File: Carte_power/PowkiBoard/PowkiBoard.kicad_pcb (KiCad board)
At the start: 4 copper layers, 74.5 x 85.5 mm, 117 parts, among them J1 AUConn, J2 VBATT, J3 GNDBATT, J4 POW_strat, J5 POW_motors, J6 POW_Access, J7 POW_access, J8 SWLogic, J9 POW_EN, Q2 DMG1012T, Q3 DMG1012T, Q4 DMG1012T, Q5 DMG1012T

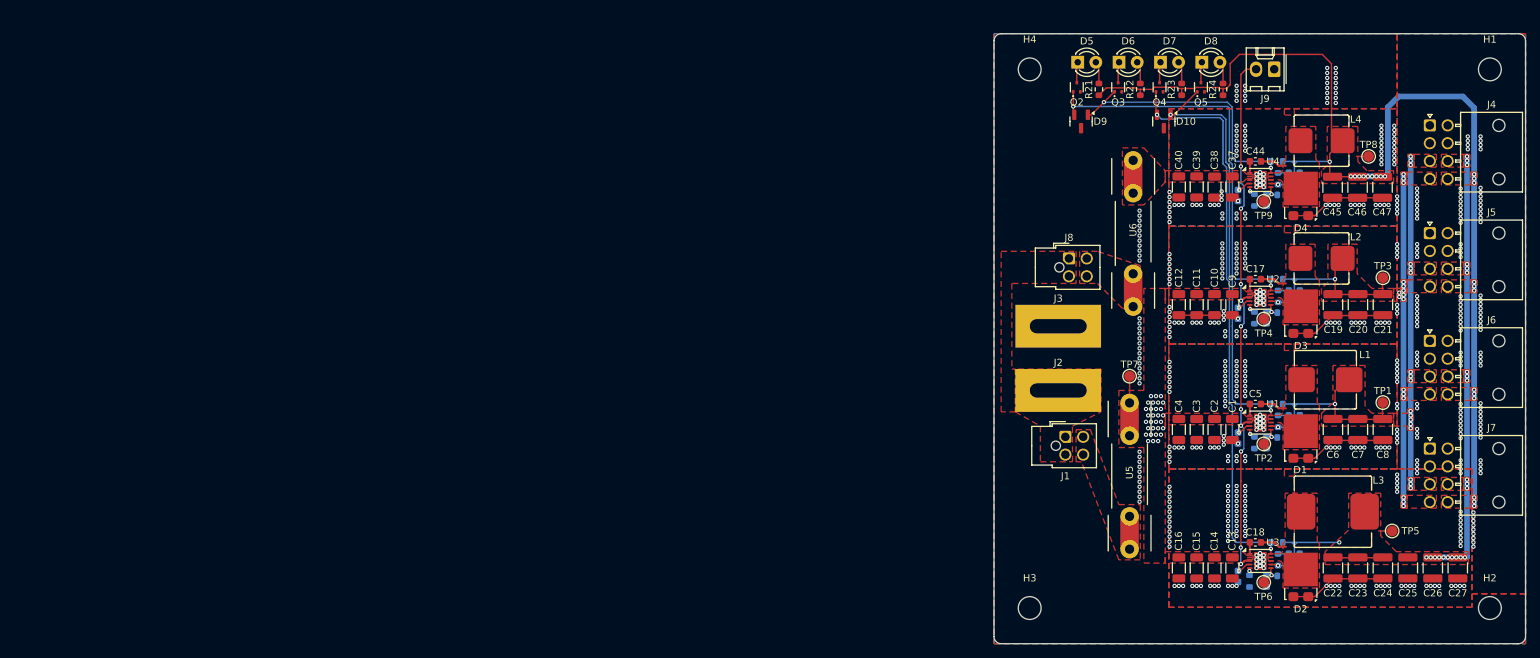
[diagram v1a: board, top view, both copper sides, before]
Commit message: AAAAAAAAAAAAAAAA
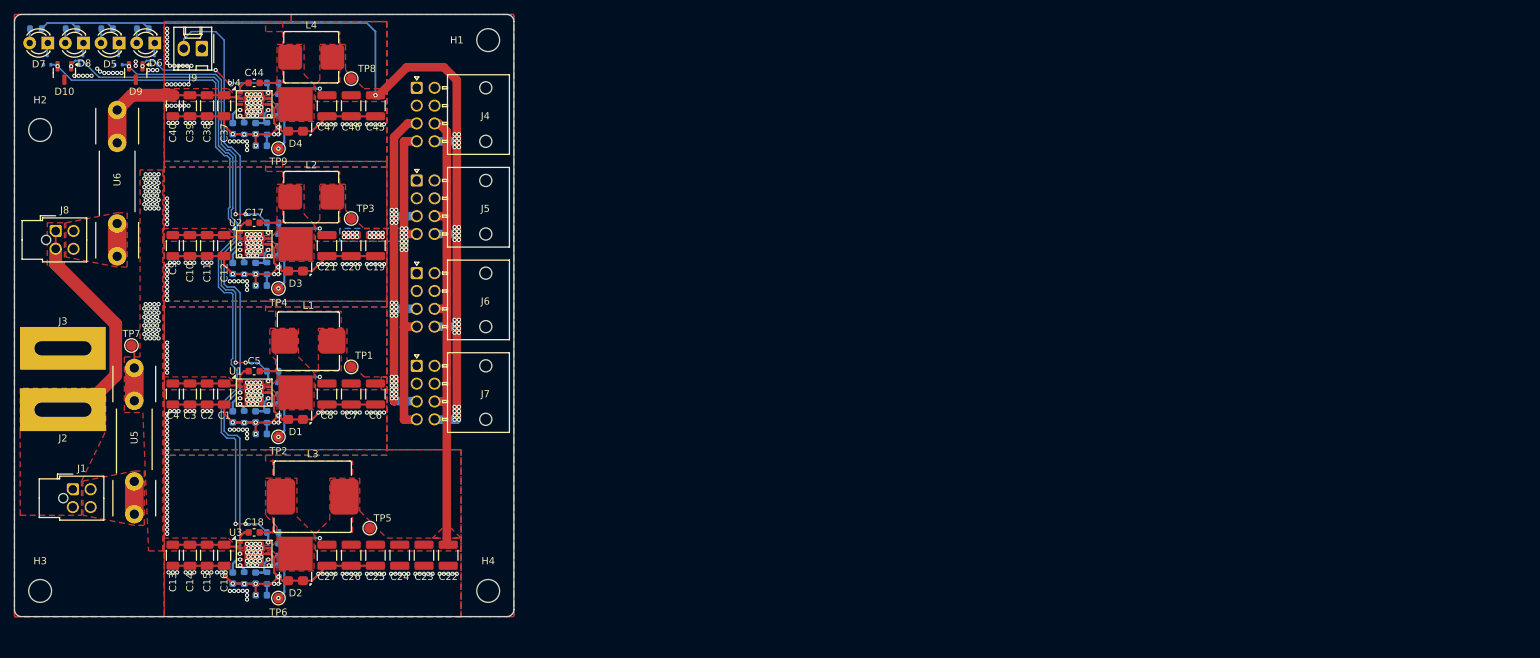
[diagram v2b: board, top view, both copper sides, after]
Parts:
- Q2, Q3, Q4, Q5, R21, R22, R23, R24: moved to B.Cu
- U1, U2, U3, U4: footprint Package_DFN_QFN:WDFN-10-1EP_3x3mm_P0.5mm_EP1.8x2.5mm -> Devices:RTQ6365
- moved H2 214.0 mm to (26.8, 60.0)
- moved R24 161.6 mm to (31.2, 45.8), turned to 180 degrees
- moved R23 160.8 mm to (26.2, 45.8), turned to 180 degrees
- moved C27 158.5 mm to (67.0, 119.6)
- moved D8 156.8 mm to (32.9, 47.8), turned to 180 degrees
- moved Q5 156.7 mm to (32.8, 50.2)
- moved D7 156.0 mm to (27.9, 47.8), turned to 180 degrees
- moved Q4 155.9 mm to (27.8, 50.2)
- moved D10 154.2 mm to (30.2, 52.0)
- moved C26 151.6 mm to (70.4, 119.6)
- moved J9 150.3 mm to (49.5, 48.6)
- moved C9 148.7 mm to (45.4, 76.2)
- moved C13 148.5 mm to (45.4, 119.6)
- moved C47 148.4 mm to (67.0, 56.6)
- moved C21 148.2 mm to (67.0, 76.2)
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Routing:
- net GNDA: track 67.6 -> 170.3 mm, vias 558 -> 359
- net VIN: track 190.7 -> 147.2 mm, vias 30 -> 72
- net VBATT: track 0.00 -> 33.5 mm
- net PG12V: track 79.7 -> 98.9 mm, vias 2 -> 4
- net Net-(U4-VIN): track 0.00 -> 18.3 mm
- net PGLG5V: track 37.7 -> 20.7 mm, vias 2 -> 4
- net 5V: track 73.8 -> 58.5 mm, vias 17 -> 29
- net PG5V: track 56.2 -> 41.0 mm, vias 2 -> 4
- net LG5V: track 162.2 -> 150.4 mm, vias 22 -> 34
- net PG9V: track 60.3 -> 71.9 mm, vias 2 -> 4
- net EN12V: track 76.7 -> 86.5 mm, vias 10 -> 3
- net 12V: track 84.3 -> 75.0 mm, vias 23 -> 1
- net 9V: track 73.8 -> 66.6 mm, vias 18 -> 29
- net Net-(U3-FB): track 4.10 -> 8.01 mm, vias 1 -> 2
- net Net-(U2-FB): track 4.10 -> 8.01 mm, vias 1 -> 2
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- removed copper zone on B.Cu, net 12V
- removed copper zone on B.Cu, net 9V
- removed copper zone on B.Cu, net LG5V
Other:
- board size 74.5 x 85.5 mm -> 70 x 84.4 mm
